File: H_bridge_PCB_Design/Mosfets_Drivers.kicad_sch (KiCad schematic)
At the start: 49 parts, among them J2 TSW-102-15-T-S, J3 TSW-102-15-T-S, J6 TSW-102-15-T-S, J7 TSW-102-15-T-S, J9 TSW-102-15-T-S, Q1 IRLB4030PBF, Q10 IPD90N10S4L06ATMA1, Q2 IRLB4030PBF, Q3 IRLB4030PBF, Q4 IRLB4030PBF, Q5 IPD90N10S4L06ATMA1, Q6 IPD90N10S4L06ATMA1, Q9 IPD90N10S4L06ATMA1, U2 IR2110S, U3 IR2110S

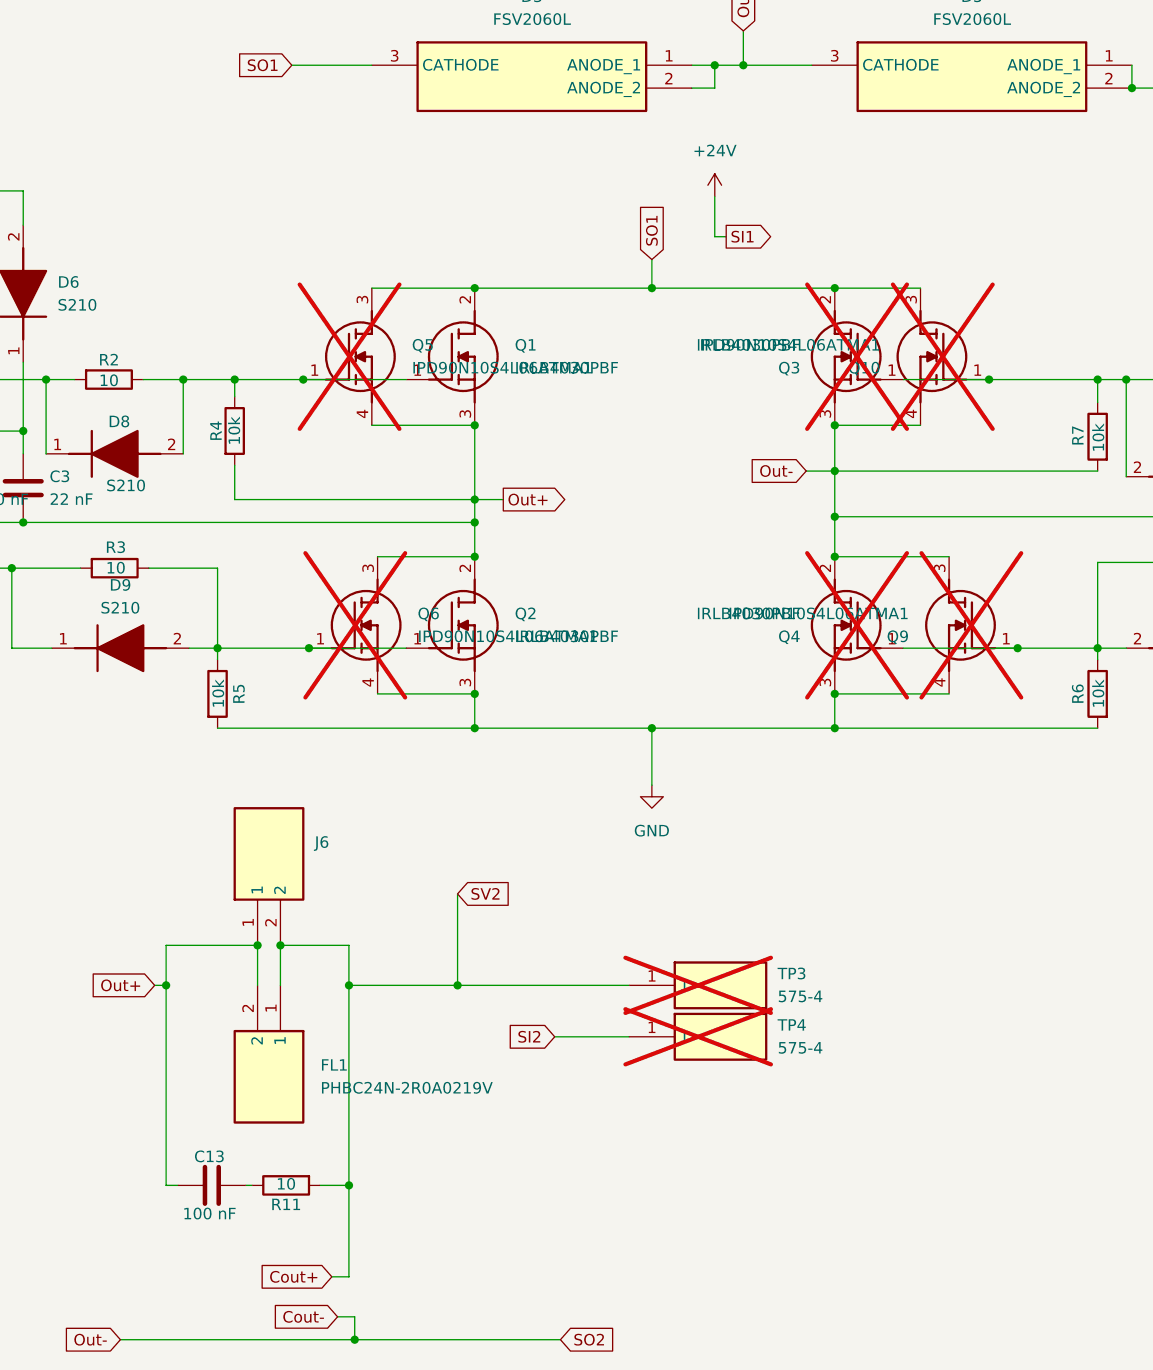
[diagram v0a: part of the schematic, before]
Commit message: huge changes output measurement
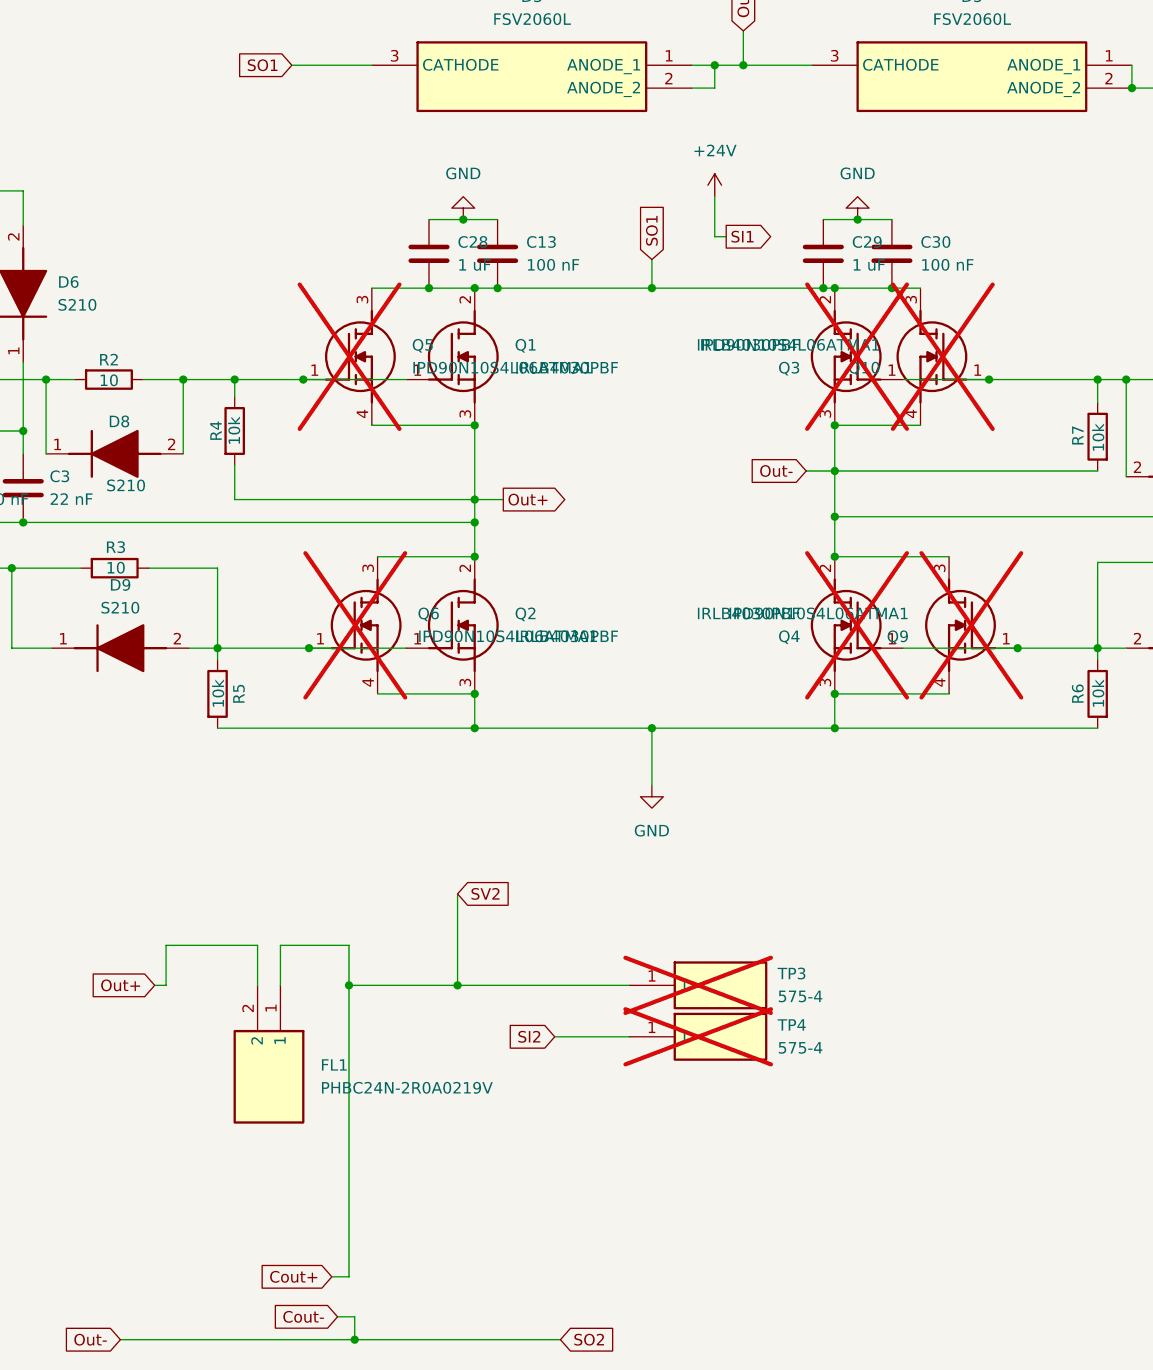
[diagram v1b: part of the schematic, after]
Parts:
- removed J6: TSW-102-15-T-S, SamacSys_Parts:TSW-102-XX-YY-S, symbol SamacSys_Parts:TSW-102-15-T-S
- removed R11: 10, Resistor_SMD:R_0805_2012Metric_Pad1.20x1.40mm_HandSolder, symbol Device:R
- added C28, C29: 1 uF, Resistor_SMD:R_0805_2012Metric_Pad1.20x1.40mm_HandSolder, symbol Device:C
- added C30: 100 nF, Resistor_SMD:R_0805_2012Metric_Pad1.20x1.40mm_HandSolder, symbol Device:C
- C13: LCSC Part# C354366 -> C513763
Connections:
- net GND: now also C13.2, C28.2, C29.2, C30.2
- net Out+: no longer C13.2
- net SO1: now also C13.1, C28.1, C29.1, C30.1
